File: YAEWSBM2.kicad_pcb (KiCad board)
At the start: 2 copper layers, 19.5 x 23.5 mm, 21 parts, among them J1 Conn_01x01_Pin, J2 Conn_01x01_Pin, J3 Conn_01x08_Pin, Q1 MMBT3904, Q2 MMBT3904

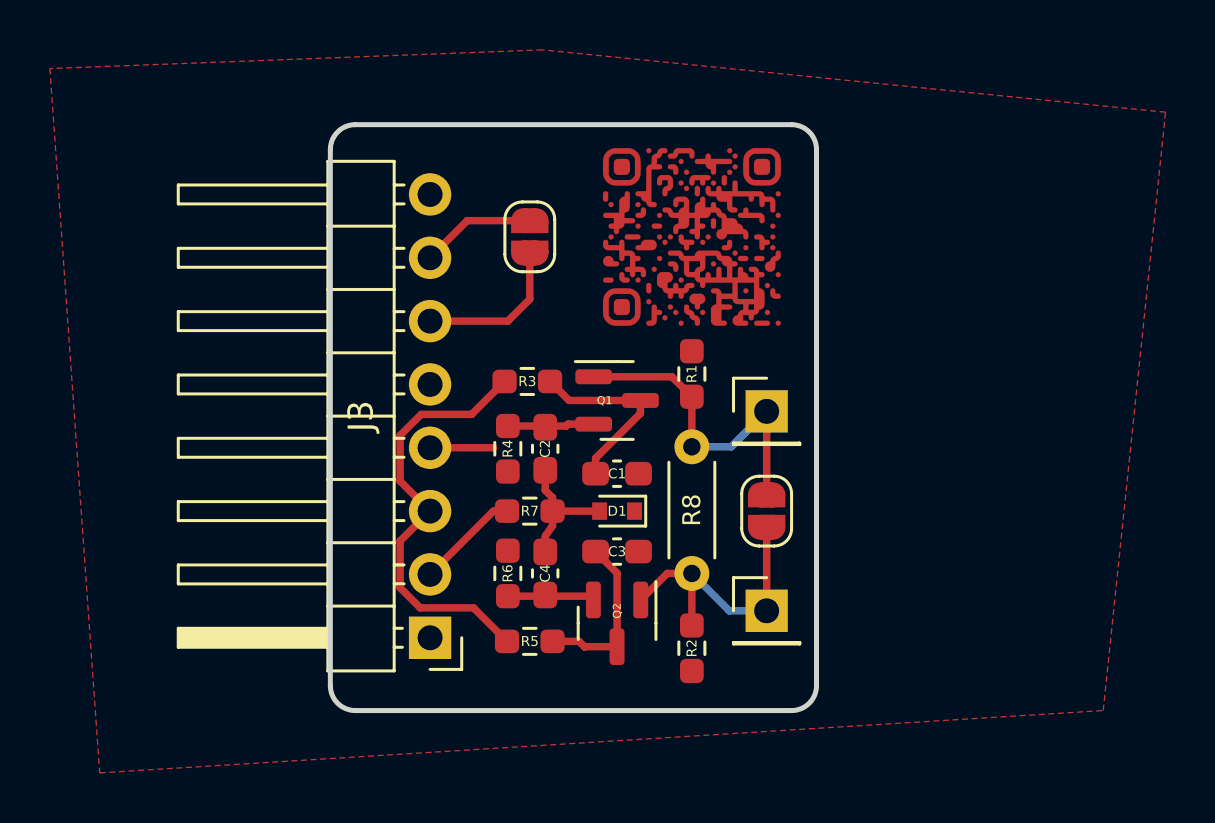
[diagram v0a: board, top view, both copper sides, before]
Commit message: silk art
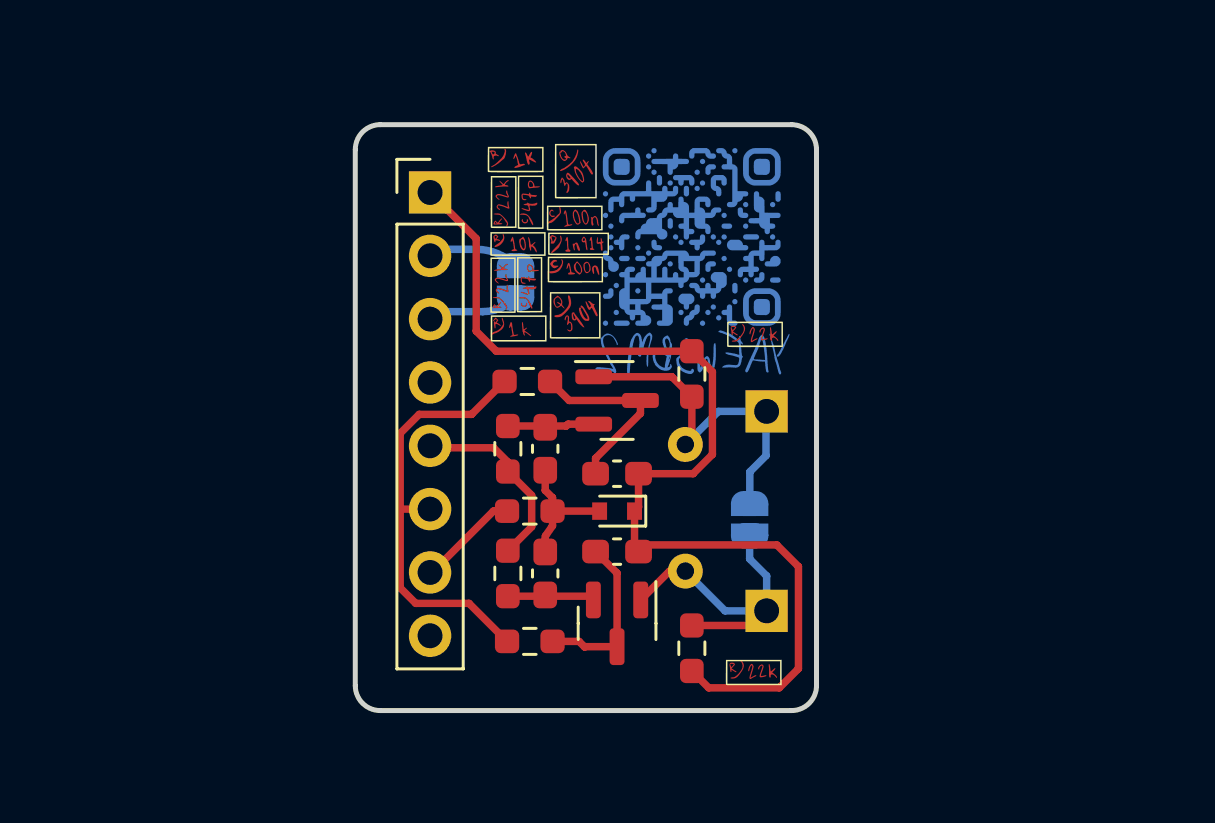
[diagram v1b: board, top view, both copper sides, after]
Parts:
- added ?: , YAEWSBM2:rearcopper, B.Cu at (109.6, 86.5)
- added G***: LOGO, YAEWSBM2:frontmask, F.Cu at (109.5, 86.5)
- added G***: LOGO, YAEWSBM2:frontsilk, F.Cu at (109.5, 86.5)
- added G***: LOGO, YAEWSBM2:frontcopper, F.Cu at (109.5, 86.5)
- added G***: LOGO, YAEWSBM2:rearsilk, B.Cu at (109.6, 86.4)
- G***, J1, J2, JP1, JP2, R8: moved to B.Cu
- J3: footprint Connector_PinHeader_2.54mm:PinHeader_1x08_P2.54mm_Horizontal -> Connector_PinHeader_2.54mm:PinHeader_1x08_P2.54mm_Vertical
- moved J3 17.9 mm to (103.5, 77.7), turned to 0 degrees
- moved JP2 1.89 mm to (106.9, 81.3)
- moved JP1 0.77 mm to (116.3, 90.8)
- moved R8 0.28 mm to (113.7, 92.9)
- turned G*** to 180 degrees
- turned J1 to 180 degrees
- turned J2 to 180 degrees
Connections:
- J3 pad 1: /AUX -> GND
- J3 pad 2: /AUDIO -> /VCA_OUT
- J3 pad 3: +12V -> /AMP_IN
- J3 pad 4: -12V -> /AMP_OUT
- J3 pad 5: /AMP_OUT -> -12V
- J3 pad 6: /AMP_IN -> +12V
- J3 pad 7: /VCA_OUT -> /AUDIO
- J3 pad 8: GND -> /AUX
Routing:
- net GND: track 0.00 -> 42.2 mm
- net -12V: track 2.55 -> 7.70 mm
- net /AMP_IN: track 6.21 -> 3.64 mm
- net Net-(J2-Pin_1): track 11.5 -> 12.7 mm
- net /VCA_OUT: track 4.62 -> 3.66 mm
- net Net-(J1-Pin_1): track 13.4 -> 14.1 mm
- removed copper zone on F.Cu, net GND
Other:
- board size 19.5 x 23.5 mm -> 18.5 x 23.5 mm
